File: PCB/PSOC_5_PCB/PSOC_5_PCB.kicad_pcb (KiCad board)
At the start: 2 copper layers, 86.6 x 56.7 mm, 63 parts, among them IC1 CY8C5888LTI-LP097, J1 USB_B_Micro, J10 GPIO Pins 7, J11 GPIO Pins 6, J12 GPIO Pins 2, J13 GPIO Pins 3, J14 GPIO Pins 5, J16 GPIO Pins 4, J2 Program Upload Interface, J3 Debug Print Interface, J4 RPI UART, J5 OEM UART, J6 Pressure Before ΔΣ, J7 SAR ADC, J8 Pressure After ΔΣ, J9 GPIO Pins 1, SW1 RESET_BUTTON

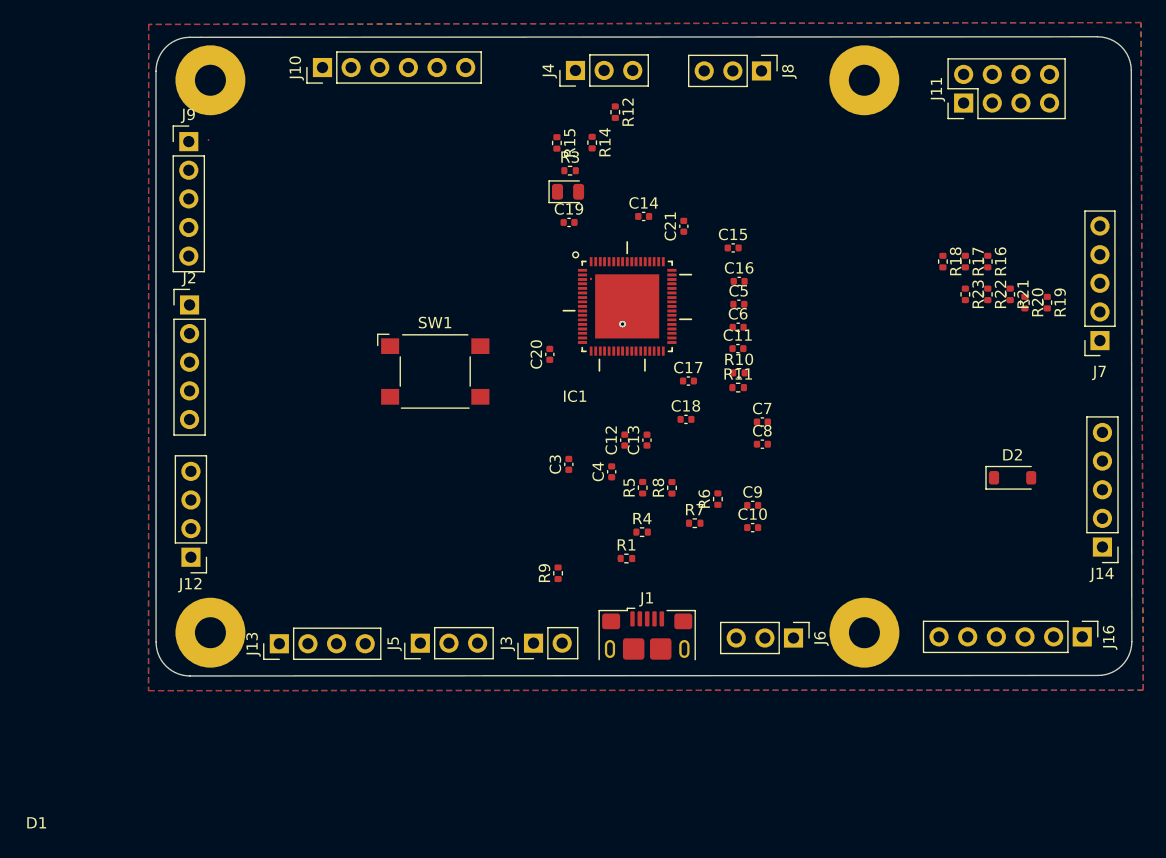
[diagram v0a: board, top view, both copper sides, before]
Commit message: PCB Layout Pushed
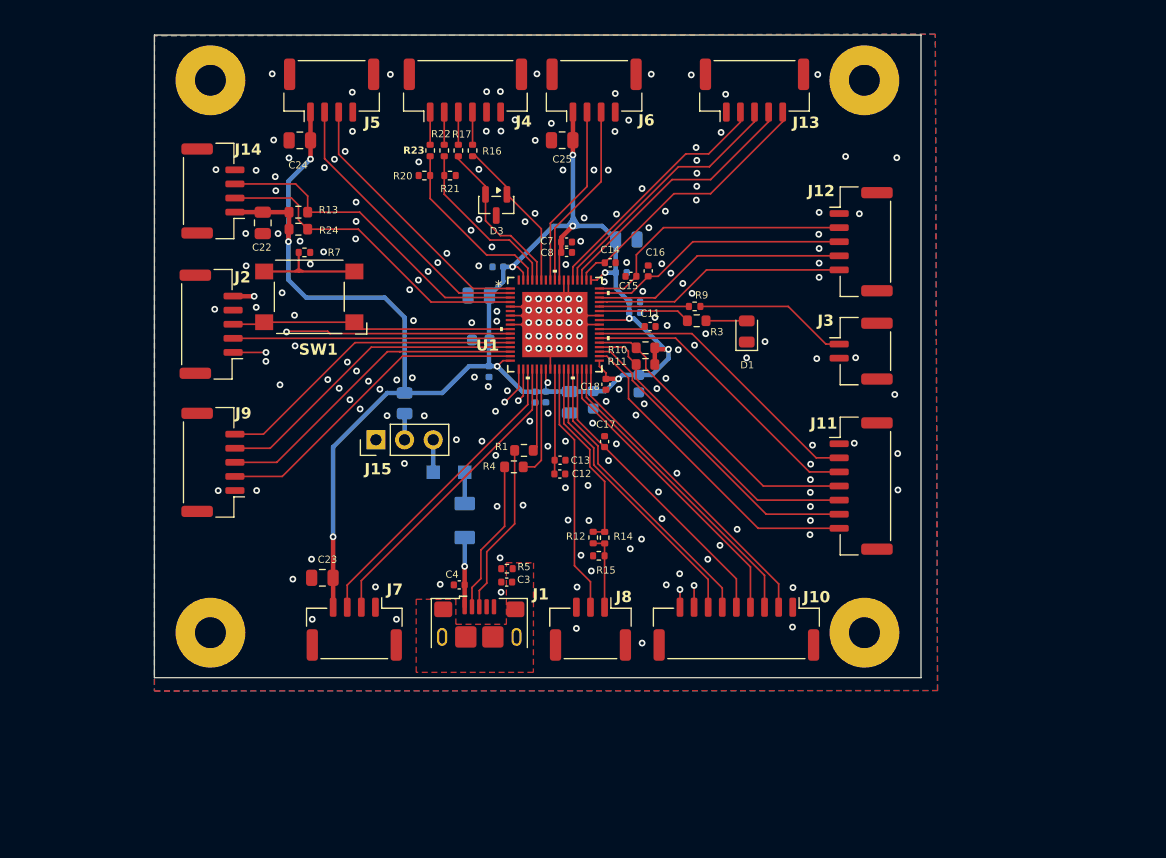
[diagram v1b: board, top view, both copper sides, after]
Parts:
- removed IC1: CY8C5888LTI-LP097, CY8C5888LTI-LP097:QFN40P800X800X100-69N
- removed J16: GPIO Pins 4, Connector_PinHeader_2.54mm:PinHeader_1x06_P2.54mm_Vertical
- removed R18, R19: 10KΩ, Resistor_SMD:R_0402_1005Metric
- removed R8: 0Ω, Resistor_SMD:R_0402_1005Metric
- added C22: 10uF, Capacitor_SMD:C_0805_2012Metric, F.Cu at (109.1, 104.6)
- added C23: 10uF, Capacitor_SMD:C_0805_2012Metric, F.Cu at (114.4, 136.0)
- added C24: 10uF, Capacitor_SMD:C_0805_2012Metric, F.Cu at (112.4, 97.2)
- added C25: 10uF, Capacitor_SMD:C_0805_2012Metric, F.Cu at (135.7, 97.2)
- added C26: 10uF, Capacitor_SMD:C_0805_2012Metric, B.Cu at (141.4, 106.0)
- added C28: 10uF, Capacitor_SMD:C_0805_2012Metric, B.Cu at (136.4, 120.5)
- added C29: 10uF, Capacitor_SMD:C_0805_2012Metric, B.Cu at (128.3, 111.0)
- added C30: 1uF, Capacitor_SMD:C_0603_1608Metric, B.Cu at (142.5, 118.8)
- added C31: 1uF, Capacitor_SMD:C_0603_1608Metric, B.Cu at (138.4, 120.3)
- added C32: 1uF, Capacitor_SMD:C_0603_1608Metric, B.Cu at (128.4, 115.0)
- added D3: D_Schottky_KKA, Package_TO_SOT_SMD:SOT-23, F.Cu at (129.8, 103.0)
- added F1: Polyfuse, ECMO:RESC3216X125N, B.Cu at (127.0, 131.0)
- added J15: Power Jumper, Connector_PinHeader_2.54mm:PinHeader_1x03_P2.54mm_Vertical, F.Cu at (119.2, 123.8)
- added R13: 4.7KΩ, Resistor_SMD:R_0603_1608Metric, F.Cu at (112.3, 103.6)
- added R24: 4.7KΩ, Resistor_SMD:R_0603_1608Metric, F.Cu at (112.3, 105.1)
- added U1: CY8C5888LTI-LP097, ECMO:QFN-68, F.Cu at (135.0, 113.6)
- C10, C19, C20, C21, C5, C6, C9: moved to B.Cu
- D2: value SOD123 -> PMEG2010ER; footprint Diode_SMD:D_SOD-123 -> Diode_SMD:Nexperia_CFP3_SOD-123W; moved to B.Cu
- J10: value GPIO Pins 7 -> GPIO_2; footprint Connector_PinHeader_2.54mm:PinHeader_1x06_P2.54mm_Vertical -> Connector_JST:JST_GH_BM09B-GHS-TBT_1x09-1MP_P1.25mm_Vertical
- J11: value GPIO Pins 6 -> GPIO_3; footprint Connector_PinHeader_2.54mm:PinHeader_2x04_P2.54mm_Vertical -> Connector_JST:JST_GH_BM07B-GHS-TBT_1x07-1MP_P1.25mm_Vertical
- J12: value GPIO Pins 2 -> GPIO_4; footprint Connector_PinHeader_2.54mm:PinHeader_1x04_P2.54mm_Vertical -> Connector_JST:JST_GH_BM05B-GHS-TBT_1x05-1MP_P1.25mm_Vertical
- J13: value GPIO Pins 3 -> GPIO_5; footprint Connector_PinHeader_2.54mm:PinHeader_1x04_P2.54mm_Vertical -> Connector_JST:JST_GH_BM05B-GHS-TBT_1x05-1MP_P1.25mm_Vertical
- J14: value GPIO Pins 5 -> I2C_1; footprint Connector_PinHeader_2.54mm:PinHeader_1x05_P2.54mm_Vertical -> Connector_JST:JST_GH_BM04B-GHS-TBT_1x04-1MP_P1.25mm_Vertical
- J2: value Program Upload Interface -> Program_Upload_Interface; footprint Connector_PinHeader_2.54mm:PinHeader_1x05_P2.54mm_Vertical -> Connector_JST:JST_GH_BM05B-GHS-TBT_1x05-1MP_P1.25mm_Vertical
- J3: value Debug Print Interface -> Debug_Interface; footprint Connector_PinHeader_2.54mm:PinHeader_1x02_P2.54mm_Vertical -> Connector_JST:JST_GH_BM02B-GHS-TBT_1x02-1MP_P1.25mm_Vertical
- J4: value RPI UART -> SAR_ADC; footprint Connector_PinHeader_2.54mm:PinHeader_1x03_P2.54mm_Vertical -> Connector_JST:JST_GH_BM06B-GHS-TBT_1x06-1MP_P1.25mm_Vertical
- J5: value OEM UART -> ΔΣ Pressure Before Gas Exchange; footprint Connector_PinHeader_2.54mm:PinHeader_1x03_P2.54mm_Vertical -> Connector_JST:JST_GH_BM04B-GHS-TBT_1x04-1MP_P1.25mm_Vertical
- J6: value Pressure Before ΔΣ -> ΔΣ Pressure After Gas Exchange; footprint Connector_PinHeader_2.54mm:PinHeader_1x03_P2.54mm_Vertical -> Connector_JST:JST_GH_BM04B-GHS-TBT_1x04-1MP_P1.25mm_Vertical
- J7: value SAR ADC -> OEM_UART; footprint Connector_PinSocket_2.54mm:PinSocket_1x05_P2.54mm_Vertical -> Connector_JST:JST_GH_BM04B-GHS-TBT_1x04-1MP_P1.25mm_Vertical
- J8: value Pressure After ΔΣ -> RPI UART; footprint Connector_PinHeader_2.54mm:PinHeader_1x03_P2.54mm_Vertical -> Connector_JST:JST_GH_BM03B-GHS-TBT_1x03-1MP_P1.25mm_Vertical
- J9: value GPIO Pins 1 -> GPIO_1; footprint Connector_PinHeader_2.54mm:PinHeader_1x05_P2.54mm_Vertical -> Connector_JST:JST_GH_BM05B-GHS-TBT_1x05-1MP_P1.25mm_Vertical
- R1, R10, R11, R3, R4: footprint Resistor_SMD:R_0402_1005Metric -> Resistor_SMD:R_0603_1608Metric
- R12: value 0Ω -> 0Ω(DNI)
- R14: value 10KΩ -> 5KΩ
- R15: value 20KΩ -> 10KΩ
- R22, R23: value 10KΩ -> 2.2KΩ
- R6: footprint Resistor_SMD:R_0402_1005Metric -> Resistor_SMD:R_0805_2012Metric; moved to B.Cu
- R7: value 0Ω -> 1KΩ
- moved J14 85.0 mm to (104.7, 101.7), turned to 90 degrees
- moved J7 70.9 mm to (117.2, 140.6)
- moved J12 65.7 mm to (162.2, 106.2), turned to -90 degrees
- moved J13 64.7 mm to (152.7, 92.8), turned to 0 degrees
- moved J10 61.9 mm to (151.1, 140.6), turned to 180 degrees
- moved R20 54.4 mm to (123.5, 100.4), turned to 0 degrees
- moved J8 51.8 mm to (138.2, 140.6), turned to 180 degrees
- moved J6 51.7 mm to (138.5, 92.8), turned to 0 degrees
- moved R21 50.8 mm to (125.7, 100.4), turned to 180 degrees
- moved D2 50.0 mm to (125.6, 126.7)
- moved R22 49.9 mm to (125.2, 98.1)
- moved J5 49.7 mm to (115.2, 92.8), turned to 0 degrees
- moved R23 49.2 mm to (124.0, 98.1)
- moved R16 46.7 mm to (127.7, 98.1), turned to 90 degrees
- moved R17 46.0 mm to (126.5, 98.1), turned to 90 degrees
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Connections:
- ? pad S2: SHIELD -> (no net)
- ? pad S1: SHIELD -> (no net)
- ? pad S4: SHIELD -> (no net)
- ? pad S3: SHIELD -> (no net)
- C18 pad 1: /Main Microcontroller/VDDIO -> /Main Microcontroller/VDD
- C19 pad 1: /Main Microcontroller/VDDIO -> /Main Microcontroller/VDD
- C20 pad 1: /Main Microcontroller/VDDIO -> /Main Microcontroller/VDD
- C21 pad 1: /Main Microcontroller/VDDIO -> /Main Microcontroller/VDD
- C3 pad 1: Earth GND -> USB_SHIELD
- D2 pad 1: /Main Microcontroller/VTARG -> /Main Microcontroller/VBUS
- J10 pad 2: /Main Microcontroller/P2.5 -> /Main Microcontroller/P3.5
- J10 pad 3: /Main Microcontroller/P2.4 -> /Main Microcontroller/P3.4
- J10 pad 4: /Main Microcontroller/P2.3 -> /Main Microcontroller/P3.3
- J10 pad 5: /Main Microcontroller/P2.2 -> /Main Microcontroller/P3.2
- J10 pad 6: /Main Microcontroller/P2.0 -> /Main Microcontroller/P3.1
- J11 pad 2: /Main Microcontroller/P0.6 -> /Main Microcontroller/P15.3
- J11 pad 3: /Main Microcontroller/P0.2 -> /Main Microcontroller/P15.2
- J11 pad 4: /Main Microcontroller/P0.3 -> /Main Microcontroller/SDA1
- J11 pad 5: /Main Microcontroller/P0.0 -> /Main Microcontroller/SCL1
- J11 pad 6: /Main Microcontroller/P0.1 -> /Main Microcontroller/P3.7
- J11 pad 7: /Main Microcontroller/P12.2 -> /Main Microcontroller/P3.6
- J12 pad 2: /Main Microcontroller/P1.0 -> /Main Microcontroller/P0.3
- J12 pad 3: /Main Microcontroller/P1.1 -> /Main Microcontroller/P0.2
- J12 pad 4: /Main Microcontroller/P1.2 -> /Main Microcontroller/P0.1
- J13 pad 2: /Main Microcontroller/P1.3 -> /Main Microcontroller/P0.7
- J13 pad 3: /Main Microcontroller/P1.4 -> /Main Microcontroller/P0.6
- J13 pad 4: /Main Microcontroller/P1.5 -> /Main Microcontroller/P0.5
- J14 pad 1: GND -> /Main Microcontroller/VDD
- J14 pad 2: /Main Microcontroller/P3.6 -> /Main Microcontroller/SDA2
- J14 pad 3: /Main Microcontroller/I2C_SCL -> /Main Microcontroller/SCL2
- J14 pad 4: /Main Microcontroller/I2C_SDA -> GND
- J2 pad 1: /Main Microcontroller/P1.0 -> /Main Microcontroller/PROG_SWDIO
- J2 pad 2: /Main Microcontroller/P1.1 -> /Main Microcontroller/PROG_SWDCLK
- J4 pad 1: GND -> Net-(J4-Pin_1)
- J4 pad 2: /Main Microcontroller/RX_RPI -> Net-(J4-Pin_2)
- J5 pad 1: GND -> /Main Microcontroller/VDD
- J5 pad 2: /Main Microcontroller/RX_OEM -> /Main Microcontroller/Pressure_Before_Pos
- J5 pad 3: /Main Microcontroller/TX_OEM -> /Main Microcontroller/Pressure_Before_Neg
- J6 pad 1: GND -> /Main Microcontroller/VDD
- J6 pad 2: /Main Microcontroller/Pressure_Before_Pos -> /Main Microcontroller/Pressure_After_Pos
- J6 pad 3: /Main Microcontroller/Pressure_Before_Neg -> /Main Microcontroller/Pressure_After_Neg
- J7 pad 2: Net-(J7-Pin_2) -> /Main Microcontroller/TX_OEM
- J7 pad 3: Net-(J7-Pin_3) -> /Main Microcontroller/RX_OEM
- J7 pad 4: Net-(J7-Pin_4) -> /Main Microcontroller/VDD
- J8 pad 1: GND -> Net-(J8-Pin_1)
- J8 pad 2: /Main Microcontroller/Pressure_After_Pos -> /Main Microcontroller/RX_RPI
- J8 pad 3: /Main Microcontroller/Pressure_After_Neg -> GND
- J9 pad 2: /Main Microcontroller/P2.6 -> /Main Microcontroller/P1.5
- J9 pad 3: /Main Microcontroller/P2.7 -> /Main Microcontroller/P1.4
- J9 pad 4: /Main Microcontroller/P12.4 -> /Main Microcontroller/P1.3
- J9 pad 5: /Main Microcontroller/P12.5 -> /Main Microcontroller/P1.2
- R1 pad 1: /Main Microcontroller/DP_P -> /Main Microcontroller/DP
- R1 pad 2: /Main Microcontroller/DP -> /Main Microcontroller/DP_P
- R10 pad 2: /Main Microcontroller/I2C_SDA -> /Main Microcontroller/SDA1
- R11 pad 1: /Main Microcontroller/I2C_SCL -> /Main Microcontroller/SCL1
- R12 pad 1: Net-(J4-Pin_3) -> Net-(J8-Pin_1)
- R14 pad 1: Net-(J4-Pin_3) -> Net-(J8-Pin_1)
- R15 pad 1: Net-(J4-Pin_3) -> Net-(J8-Pin_1)
- R16 pad 1: Net-(J7-Pin_2) -> /Main Microcontroller/ADC_CH0
- R16 pad 2: /Main Microcontroller/ADC_CH0 -> Net-(J4-Pin_4)
- R17 pad 1: Net-(J7-Pin_3) -> /Main Microcontroller/ADC_CH1
- R17 pad 2: /Main Microcontroller/ADC_CH1 -> Net-(J4-Pin_3)
- R20 pad 2: /Main Microcontroller/ADC_CH0 -> /Main Microcontroller/ADC_CH3
- R21 pad 2: /Main Microcontroller/ADC_CH1 -> /Main Microcontroller/ADC_CH2
- R22 pad 1: GND -> Net-(J4-Pin_2)
- R23 pad 1: GND -> Net-(J4-Pin_1)
- R4 pad 1: /Main Microcontroller/DM_P -> /Main Microcontroller/DM
- R4 pad 2: /Main Microcontroller/DM -> /Main Microcontroller/DM_P
- R5 pad 1: Earth GND -> USB_SHIELD
- R6 pad 1: /Main Microcontroller/VTARG -> Net-(J15-Pin_2)
- R6 pad 2: Net-(R6-Pad2) -> /Main Microcontroller/VDD
- R7 pad 1: Net-(R6-Pad2) -> Net-(R7-Pad1)
- R7 pad 2: /Main Microcontroller/VDD -> GND
- SW1 pad 2: GND -> Net-(R7-Pad1)
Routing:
- net /Main Microcontroller/VDD: track 0.00 -> 156.7 mm, vias 0 -> 12
- net /Main Microcontroller/SCL2: track 0.00 -> 29.4 mm
- net /Main Microcontroller/SDA2: track 0.00 -> 29.0 mm
- net /Main Microcontroller/P1.5: track 0.00 -> 28.9 mm
- net /Main Microcontroller/P3.6: track 0.00 -> 28.7 mm
- net /Main Microcontroller/P1.4: track 0.00 -> 28.5 mm
- net /Main Microcontroller/P1.6: track 0.00 -> 28.3 mm, vias 0 -> 2
- net /Main Microcontroller/P1.3: track 0.00 -> 28.1 mm
- net /Main Microcontroller/P3.5: track 0.00 -> 28.0 mm
- net /Main Microcontroller/SCL1: track 0.00 -> 27.9 mm
- net /Main Microcontroller/P1.2: track 0.00 -> 27.8 mm
- net /Main Microcontroller/P1.7: track 0.00 -> 27.8 mm, vias 0 -> 2
- net /Main Microcontroller/RX_OEM: track 0.00 -> 27.8 mm
- net /Main Microcontroller/P3.4: track 0.00 -> 27.7 mm
- net /Main Microcontroller/P3.7: track 0.00 -> 27.6 mm
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- added copper zone on In1.Cu, net GND
- added copper zone on In2.Cu, net GND
- added copper zone on F.Cu, net USB_SHIELD
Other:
- board size 86.6 x 56.7 mm -> 68 x 57 mm
- copper layers 2 -> 4
